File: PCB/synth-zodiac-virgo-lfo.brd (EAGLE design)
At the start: 76.1 x 72.4 mm, 37 parts, among them Q1 NPN, Q10 PNP, Q9 PNP, U1 TL074A, U2 LM13700

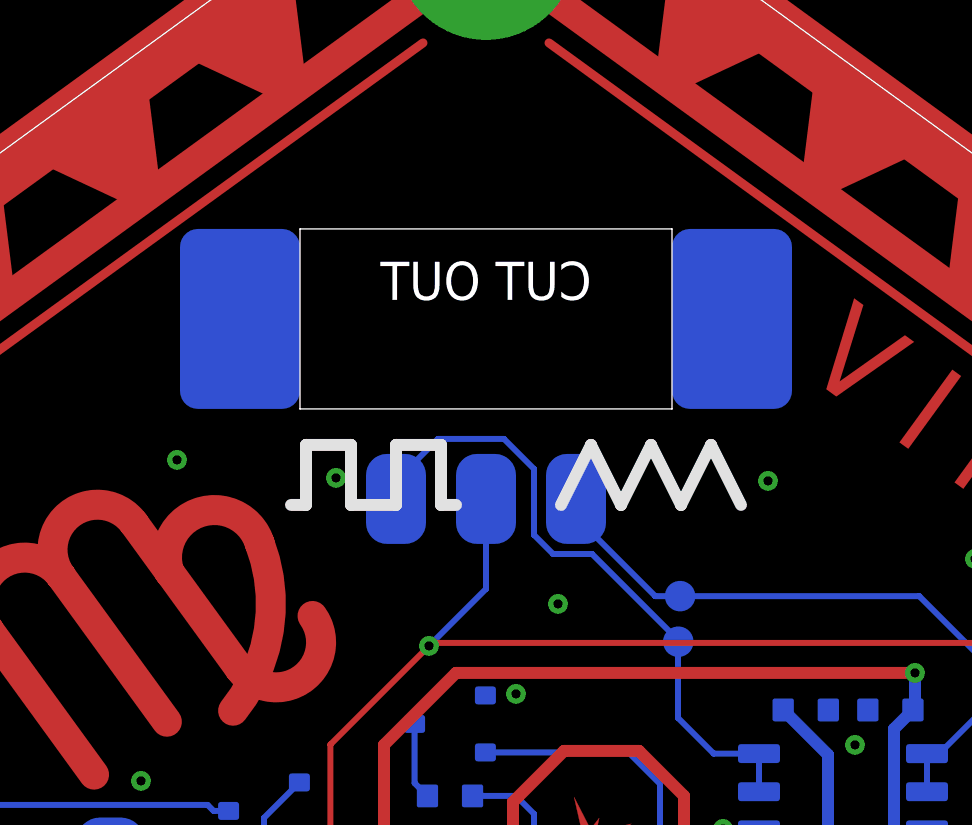
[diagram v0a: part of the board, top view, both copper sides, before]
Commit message: Perhaps final Rev. A?
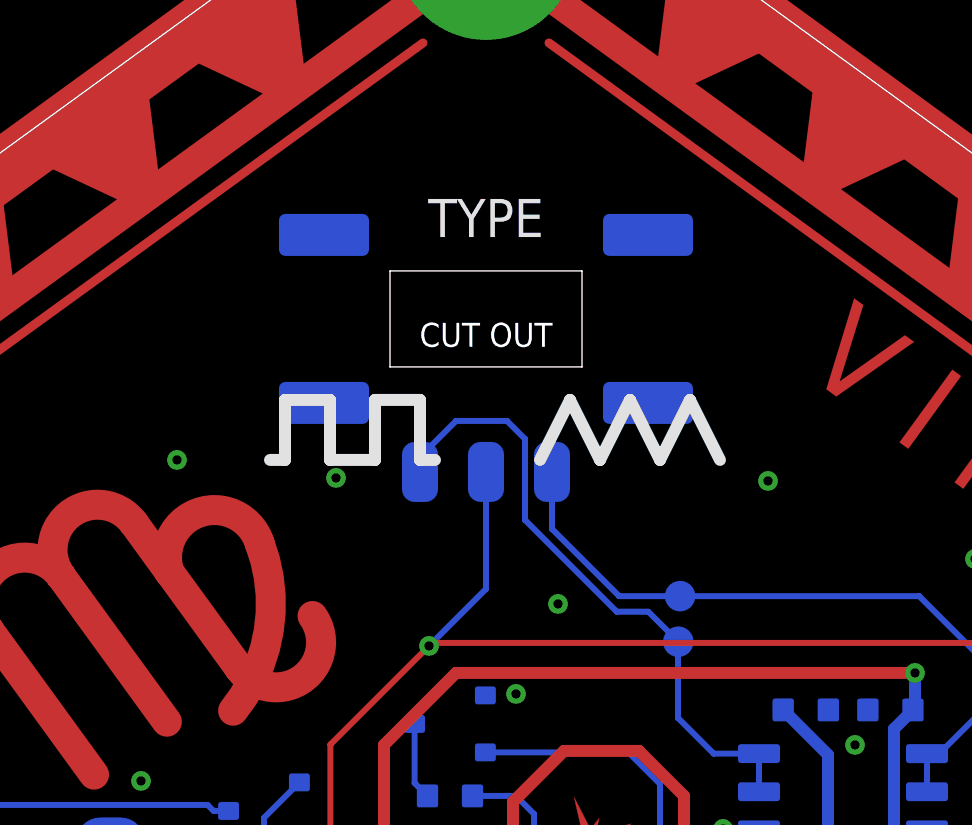
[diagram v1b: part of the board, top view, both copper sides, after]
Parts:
- TYPE: device switch-thd:SS-12-F45-PNL-SMT -> switch-thd:SS-12-F45-PNL-SMT-2
- flipped TYPE to the top
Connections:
- net LFO_SQ: now also TYPE.A; no longer TYPE.B
- net LFO_TRI: now also TYPE.B; no longer TYPE.A
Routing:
- net LFO_TRI: track 21.3 -> 23.3 mm
- net LFO_CV: track 88.2 -> 89.1 mm
